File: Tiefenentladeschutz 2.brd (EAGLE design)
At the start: 60 x 60 mm, 36 parts, among them IC1 ICL7665CSA, IC2 NE555D

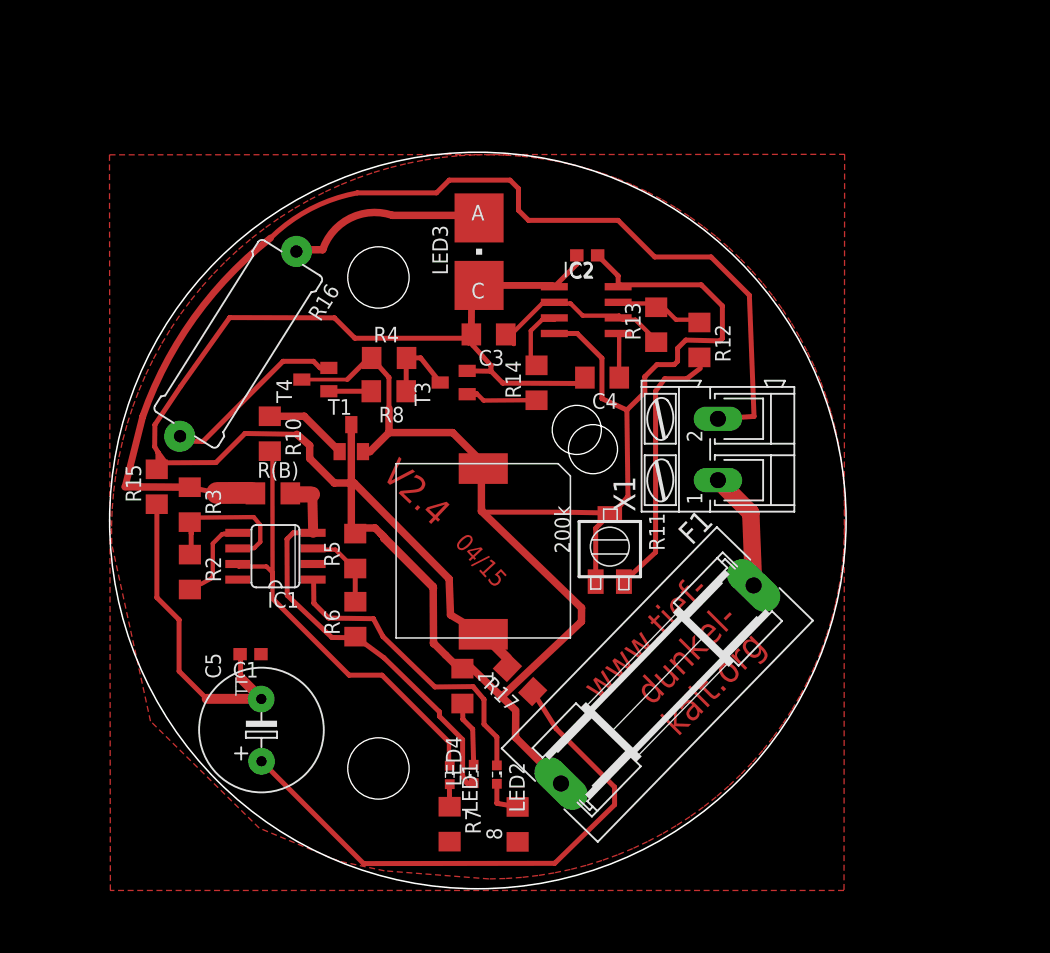
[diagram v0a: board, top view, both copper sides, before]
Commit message: 2.6
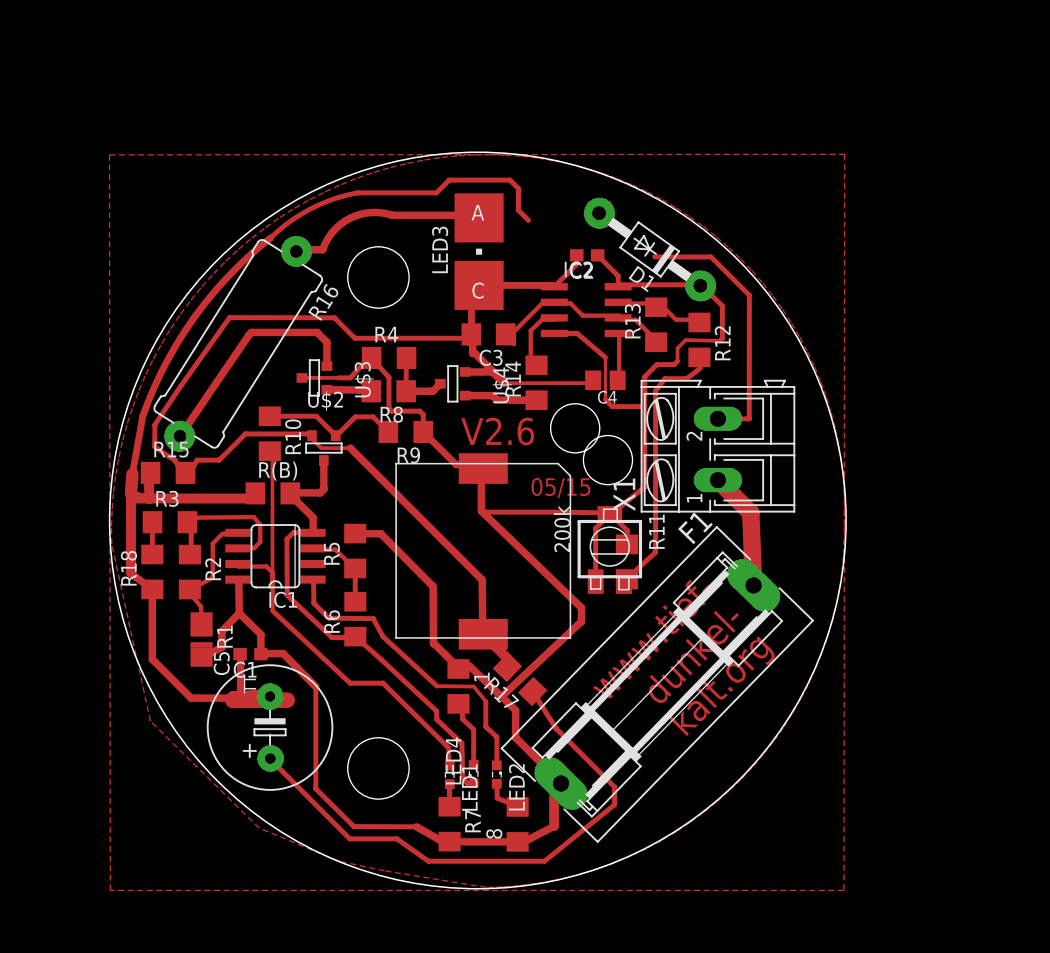
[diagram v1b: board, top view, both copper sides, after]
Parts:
- removed T1, T3, T4: (no value), transistor:SOT23-BEC
- added D1: 1N4004, diode:DO41-10
- added R1: 0, eagle-ltspice:R1206
- added R18: 5,6k, eagle-ltspice:R1206
- added R9: 100k, eagle-ltspice:R1206
- added U$2: IRLML9301, 0liver:SOT-23
- added U$3, U$4: IRLML6346, 0liver:SOT-23
- C4: value 10 nF -> 10nF; device eagle-ltspice:C1206 -> rcl:C0805K
- F1: value FUSESH22,5A -> 0,5A
- R13: value 30k -> 8,2k
- R14: value 510 -> 680
- R3: value 130k -> 120k
- R4: value ? -> 470k
- R8: value ? -> 4,7k
- moved R3 2.15 mm to (5.02, 30.1), turned to 0 degrees
- moved R15 1.46 mm to (4.86, 34.1), turned to 0 degrees
- moved C5 0.73 mm to (13.2, 13.3)
- moved C4 0.35 mm to (40.5, 41.6)
- moved 1 0.32 mm to (28.5, 16.7)
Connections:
- net GND: now also D1.A, R18.1, U$2.1; no longer R3.1
- net N$1: now also R1.1, R2.2; no longer R10.2
- net N$10: now also R10.2
- net N$17: now also U$3.3; no longer T4.B
- net N$18: now also U$4.3; no longer T3.B
- net N$21: now also U$4.1; no longer T3.C
- net N$22: now also U$2.2, U$4.2; no longer T3.E
- net N$26: now also R18.2, R3.1; no longer 1.1, 8.1, C1.1, F1.2, IC1.8, R2.2, R5.2, R7.2, T1.C
- net N$3: now also U$3.2; no longer T4.E
- net N$7: now also R9.2, U$2.3; no longer T1.B
- net V+: now also 1.1, 8.1, C1.1, D1.C, F1.2, IC1.8, R1.2, R5.2, R7.2, R9.1, U$3.1; no longer T1.E, T4.C
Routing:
- net V+: track 146.4 -> 202.8 mm
- net N$26: track 18.8 -> 2.63 mm
- net N$27: track 0.00 -> 11.3 mm
- net GND: track 155.6 -> 148.7 mm, vias 0 -> 1
- net N$7: track 6.88 -> 11.5 mm
- net N$22: track 104.0 -> 108.2 mm
- net N$1: track 6.22 -> 10.2 mm
- net N$3: track 15.6 -> 18.7 mm
- net N$30: track 0.00 -> 2.52 mm
- net N$23: track 45.9 -> 44.7 mm
- net N$10: track 38.5 -> 39.3 mm
- net N$21: track 6.42 -> 5.74 mm
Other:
- board text added: "05/15"
- board text added: "V2.6"
- board text removed: "04/15"
- board text removed: "V2.4"

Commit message: 2.7
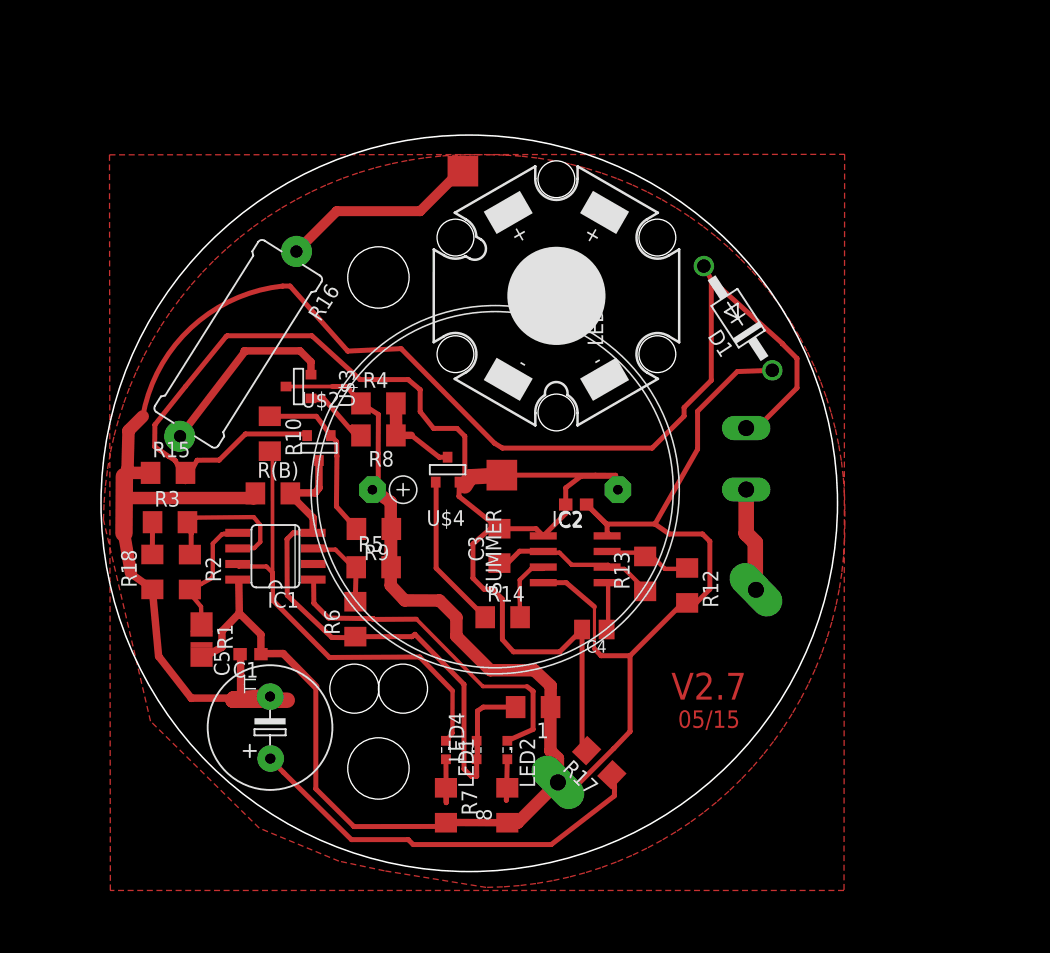
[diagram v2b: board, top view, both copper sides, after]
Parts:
- removed LED3: blue, led:P-LCC-2
- removed R11: 200k, 0liver:MINATURTRIMMER-CERMET
- added LED5: OSTAR_4-LEWE2B-MXPX-6K8L, led:OSTAR-LENS_
- SUMMER: value SUMMER -> SUMMER3; device 0liver:PIEZO-INDIKATOR-SMD-88-DB -> 0liver:PIEZO-INDIKATOR-LF-PB30P25B
- moved IC2 20.3 mm to (38.0, 27.0)
- moved C2 20.3 mm to (38.1, 31.5)
- moved C4 20.3 mm to (39.6, 21.3)
- moved R13 20.3 mm to (43.7, 25.9)
- moved R12 20.0 mm to (47.1, 24.9)
- moved R14 19.3 mm to (32.1, 22.3), turned to 0 degrees
- moved C3 17.3 mm to (31.9, 28.1), turned to 90 degrees
- moved R17 9.36 mm to (40.0, 10.5)
- moved D1 9.12 mm to (51.3, 46.7), turned to 123.3 degrees
- moved R9 8.32 mm to (21.6, 29.5)
- moved U$4 7.03 mm to (27.7, 34.3), turned to 180 degrees
- moved 1 6.31 mm to (34.6, 15.0), turned to 180 degrees
- moved SUMMER 5.07 mm to (31.5, 32.7), turned to 90 degrees
- moved R4 3.80 mm to (22.0, 39.7)
- moved R8 3.70 mm to (22.0, 37.1)
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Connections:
- removed net N$14: R11.P$3, R12.2
- removed net N$22: C2.2, C3.2, C4.2, IC2.1, LED3.C, R15.2, R17.2, SUMMER.2, U$2.2, U$4.2
- new net 2NDGND: C2.2, C3.2, C4.2, IC2.1, LED5.-, R15.2, R17.2, SUMMER.GND, U$2.2, U$4.2
- net N$12: now also LED5.+; no longer LED3.A
- net V+: now also R12.2, SUMMER.VIN; no longer R11.P$1, R11.P$2, SUMMER.1
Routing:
- net 2NDGND: track 0.00 -> 118.1 mm
- net N$22: track 108.2 -> 0.00 mm
- net V+: track 202.8 -> 175.8 mm
- net GND: track 148.7 -> 171.8 mm, vias 1 -> 0
- net N$14: track 22.0 -> 0.00 mm
- net N$23: track 44.7 -> 34.1 mm
- net N$18: track 5.96 -> 12.7 mm
- net N$11: track 25.0 -> 28.1 mm
- net N$3: track 18.7 -> 15.6 mm
- net N$6: track 1.85 -> 4.75 mm
- net N$7: track 11.5 -> 14.2 mm
- net N$17: track 3.62 -> 6.34 mm
- net N$9: track 5.62 -> 8.16 mm
- net N$30: track 2.52 -> 0.00 mm
- net N$20: track 16.8 -> 14.4 mm
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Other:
- board text added: "V2.7"
- board text removed: "V2.6"
- board text removed: "www.tief- dunkel- kalt.org"

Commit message: 3.0
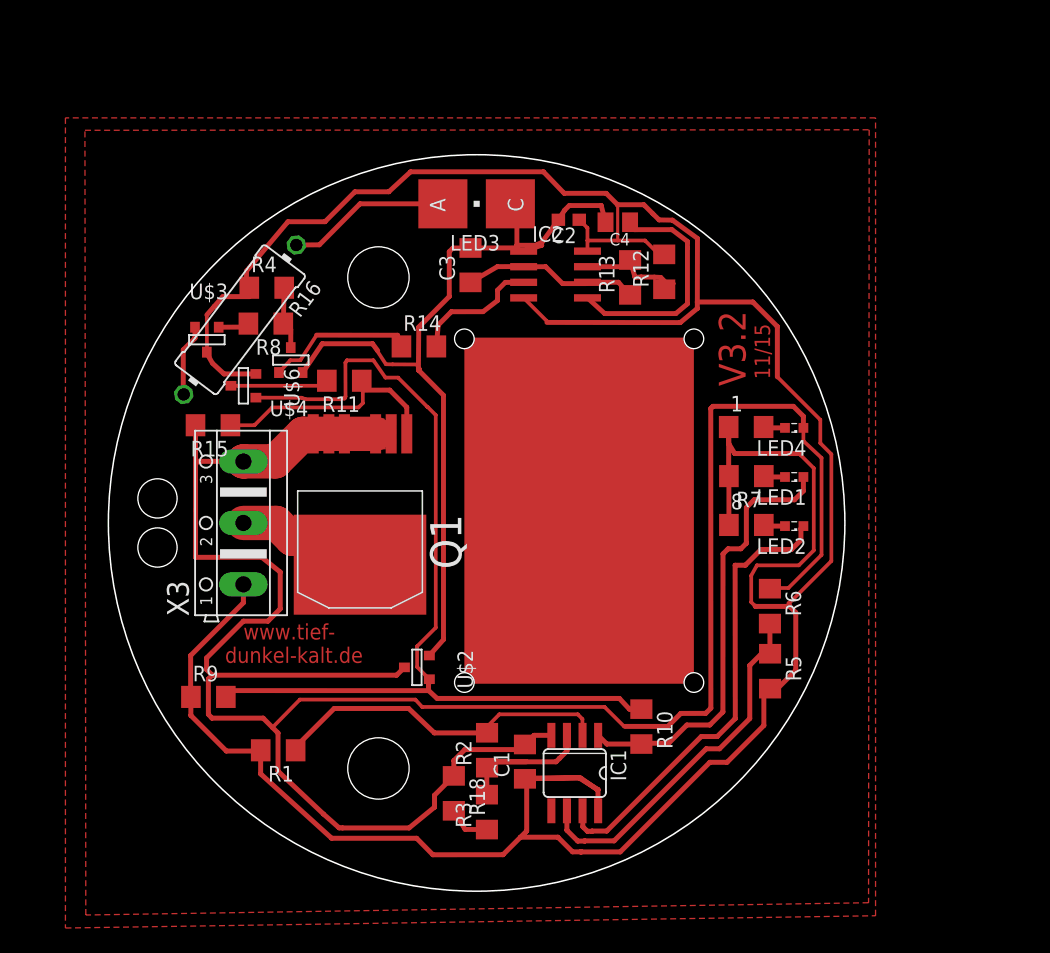
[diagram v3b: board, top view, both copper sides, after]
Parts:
- removed C5: 470 uF, rcl:TT5D10
- removed D1: 1N4004, diode:DO41-10
- removed F1: 0,5A, fuse:SH22,5A
- removed LED5: OSTAR_4-LEWE2B-MXPX-6K8L, led:OSTAR-LENS_
- removed R(B): 0 ohm, eagle-ltspice:R1206
- removed R17: 1k, eagle-ltspice:R1206
- removed SUMMER: SUMMER3, 0liver:PIEZO-INDIKATOR-LF-PB30P25B
- removed X1: (no value), con-ptr500:AK300/2
- added LED3: (no value), led:P-LCC-2
- added Q1: NMOSFET-D2PAK-7, D2pak-7:D2PAK-7
- added R11: 68k, eagle-ltspice:R1206
- added U$5: PIN-GENERIC, 0liver:LEER
- added U$6: IRLML9301, 0liver:SOT-23
- added X3: (no value), con-ptr500:AK500/3
- C1: device eagle-ltspice:C0603 -> eagle-ltspice:C1206
- LED1: value red 2mA -> green 2mA
- LED2: value green 2mA -> red 2mA
- R1: value 0 -> 100k
- R10: value 6,8 k -> 68k
- R15, R9: value 100k -> 470k
- R16: device resistor:0617/17 -> resistor:0414/15
- moved R10 38.5 mm to (43.4, 13.4)
- moved LED4 36.9 mm to (55.9, 37.7), turned to 180 degrees
- moved R7 36.3 mm to (52.0, 33.8), turned to 180 degrees
- moved LED1 36.1 mm to (55.9, 33.7), turned to 180 degrees
- moved R3 35.0 mm to (30.8, 6.44), turned to 90 degrees
- moved R6 33.8 mm to (53.9, 23.2), turned to 270 degrees
- moved R5 33.4 mm to (53.9, 17.9), turned to 270 degrees
- moved C4 33.2 mm to (41.5, 54.5)
- moved R18 30.5 mm to (28.1, 7.97), turned to 270 degrees
- moved IC1 30.1 mm to (38.0, 9.62), turned to 180 degrees
- moved 8 30.0 mm to (52.0, 29.8), turned to 0 degrees
- moved LED2 29.6 mm to (55.9, 29.7), turned to 180 degrees
- moved 1 28.7 mm to (52.0, 37.8), turned to 0 degrees
- moved R2 28.2 mm to (30.8, 11.5), turned to 90 degrees
- moved R12 25.6 mm to (45.3, 50.5), turned to 90 degrees
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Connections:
- removed net N$23: C5.+, R17.1
- removed net POWER-IN: F1.1, X1.1
- new net N$13: IC1.2, R1.1, R2.2
- new net N$16: IC1.1, LED1.C, R10.2
- new net N$22: Q1.G, R11.1, R15.1
- net 2NDGND: now also LED3.C; no longer LED5.-, R15.2, R17.2, SUMMER.GND
- net GND: now also Q1.S1, Q1.S2, Q1.S3, Q1.S4, Q1.S5, R15.2, X3.3; no longer C5.-, D1.A, R15.1, X1.2
- net N$1: now also Q1.D, X3.2; no longer IC1.5, R1.1, R2.2
- net N$10: now also R11.2, U$6.1; no longer IC1.7, LED1.C, R10.2
- net N$11: now also IC1.7; no longer IC1.1
- net N$12: now also LED3.A; no longer LED5.+
- net N$2: now also IC1.3; no longer IC1.6
- net N$4: now also IC1.6; no longer IC1.3
- net N$7: now also U$6.3
- net V+: now also U$6.2, X3.1; no longer D1.C, F1.2, SUMMER.VIN
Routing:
- net V+: track 175.8 -> 260.1 mm
- net N$7: track 14.2 -> 78.3 mm
- net 2NDGND: track 118.1 -> 70.6 mm
- net N$16: track 0.00 -> 35.9 mm, vias 1 -> 0
- net N$23: track 34.1 -> 0.00 mm
- net N$10: track 40.2 -> 8.46 mm
- net N$13: track 0.00 -> 28.1 mm, vias 1 -> 0
- net N$4: track 7.00 -> 29.8 mm
- net N$22: track 0.00 -> 20.5 mm
- net GND: track 171.8 -> 191.0 mm
- net N$19: track 3.84 -> 19.4 mm
- net N$27: track 11.0 -> 0.00 mm
- net N$3: track 15.6 -> 5.88 mm
- net N$11: track 28.1 -> 37.6 mm
- net POWER-IN: track 8.50 -> 0.00 mm
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- added copper zone on layer 1, net N$14
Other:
- board text added: "11/15"
- board text added: "V3.2"
- board text added: "www.tief- dunkel-kalt.de"
- board text removed: "05/15"
- board text removed: "V2.7"

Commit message: 3.3
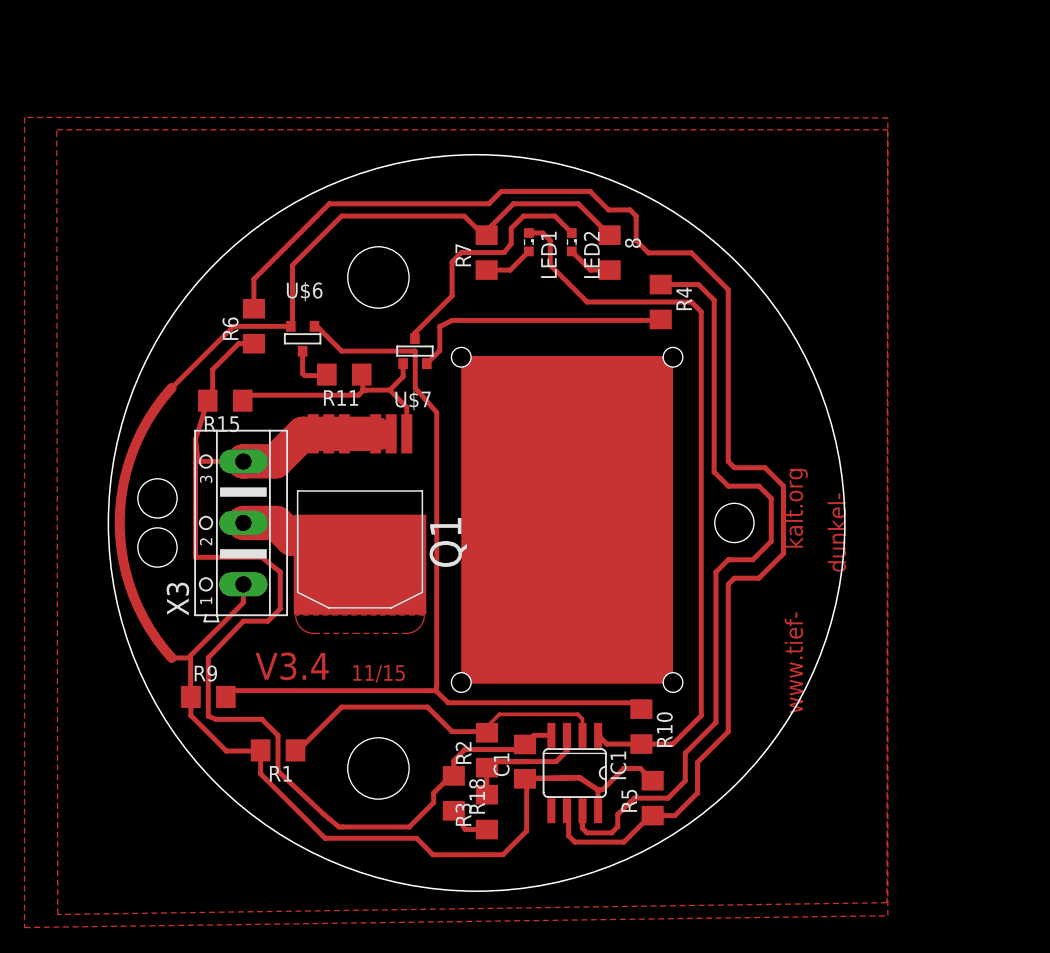
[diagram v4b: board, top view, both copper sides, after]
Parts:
- removed 1: 5,6k, eagle-ltspice:R1206
- removed C2: 100 nF, eagle-ltspice:C0603
- removed C3: 10 µF, eagle-ltspice:C1206
- removed C4: 10nF, rcl:C0805K
- removed IC2: NE555D, linear:SO08
- removed LED3: (no value), led:P-LCC-2
- removed LED4: yellow 2mA, eagle-ltspice:LED_SML0603
- removed R12: 42,2k, eagle-ltspice:R1206
- removed R13: 8,2k, eagle-ltspice:R1206
- removed R14: 680, eagle-ltspice:R1206
- removed R16: 27, resistor:0414/15
- removed R8: 4,7k, eagle-ltspice:R1206
- removed U$2: IRLML9301, 0liver:SOT-23
- removed U$3, U$4: IRLML6346, 0liver:SOT-23
- added U$7: IRLML6346, 0liver:SOT-23
- R4: value 470k -> 0
- moved R6 47.8 mm to (11.9, 46.0), turned to 90 degrees
- moved R4 32.1 mm to (45.0, 48.0), turned to 270 degrees
- moved LED2 29.4 mm to (37.8, 52.9), turned to 270 degrees
- moved LED1 28.9 mm to (34.3, 52.9), turned to 270 degrees
- moved R7 27.9 mm to (30.8, 52.0), turned to 90 degrees
- moved 8 24.8 mm to (40.8, 52.0), turned to 270 degrees
- moved R5 14.1 mm to (44.3, 7.58), turned to 90 degrees
- moved U$6 6.12 mm to (15.8, 45.0), turned to 0 degrees
- moved R15 2.24 mm to (9.52, 40.0)
- moved R11 0.50 mm to (19.2, 42.1)
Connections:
- removed net 2NDGND: C2.2, C3.2, C4.2, IC2.1, LED3.C, U$2.2, U$4.2
- removed net N$12: LED3.A, R16.1
- removed net N$15: IC2.7, R12.1, R13.2
- removed net N$17: R8.2, U$3.3
- removed net N$18: R14.1, U$4.3
- removed net N$19: C4.1, IC2.5
- removed net N$20: C3.1, IC2.2, IC2.6, R13.1
- removed net N$21: R4.2, R8.1, U$4.1
- removed net N$8: IC2.3, R14.2
- removed net N$9: 1.2, LED4.A
- new net N$23: IC1.7, R4.1
- net GND: no longer LED4.C, U$2.1
- net N$11: now also U$7.1; no longer IC1.7
- net N$22: now also U$7.3
- net N$3: now also R4.2, U$7.2; no longer R16.2, U$3.2
- net N$7: no longer U$2.3
- net V+: no longer 1.1, C2.1, IC2.4, IC2.8, R12.2, R4.1, U$3.1
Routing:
- net V+: track 260.1 -> 142.1 mm
- net GND: track 191.0 -> 104.3 mm
- net N$4: track 29.8 -> 111.4 mm
- net 2NDGND: track 70.6 -> 0.00 mm
- net N$23: track 0.00 -> 63.8 mm
- net N$16: track 35.9 -> 60.6 mm
- net N$19: track 19.4 -> 0.00 mm
- net N$11: track 37.6 -> 20.2 mm
- net N$3: track 5.88 -> 21.8 mm
- net N$20: track 14.3 -> 0.00 mm
- net N$12: track 13.3 -> 0.00 mm
- net N$18: track 12.2 -> 0.00 mm
- net N$8: track 11.0 -> 0.00 mm
- net N$15: track 10.4 -> 0.00 mm
- net N$7: track 78.3 -> 72.5 mm
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- added copper zone on layer 1, net N$1
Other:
- board text added: "V3.4"
- board text added: "dunkel-"
- board text added: "www.tief- kalt.org"
- board text removed: "V3.2"
- board text removed: "www.tief- dunkel-kalt.de"
